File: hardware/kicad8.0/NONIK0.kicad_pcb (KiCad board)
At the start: 2 copper layers, 55 x 22 mm, 24 parts, among them J1 AVR-UPDI-3, J2 Qwiic/Stemma QT, J3 Test Pads, J4 Test Pads, SW1 SW_SPST, SW2 SW_Push, SW3 SW_Push, U1 LED_HCMS-2915, U2 ATtiny1604-SS, U3 AP3602A

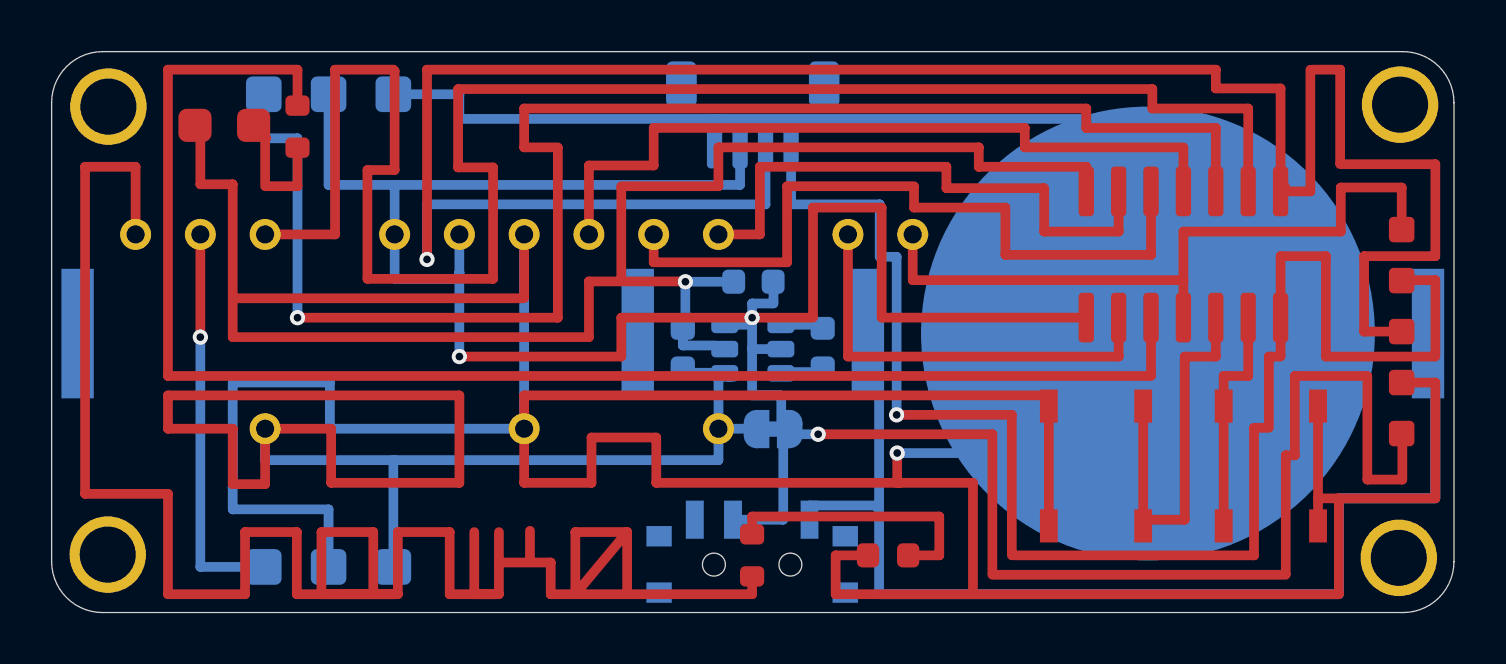
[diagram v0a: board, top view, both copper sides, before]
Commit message: pcb revisions
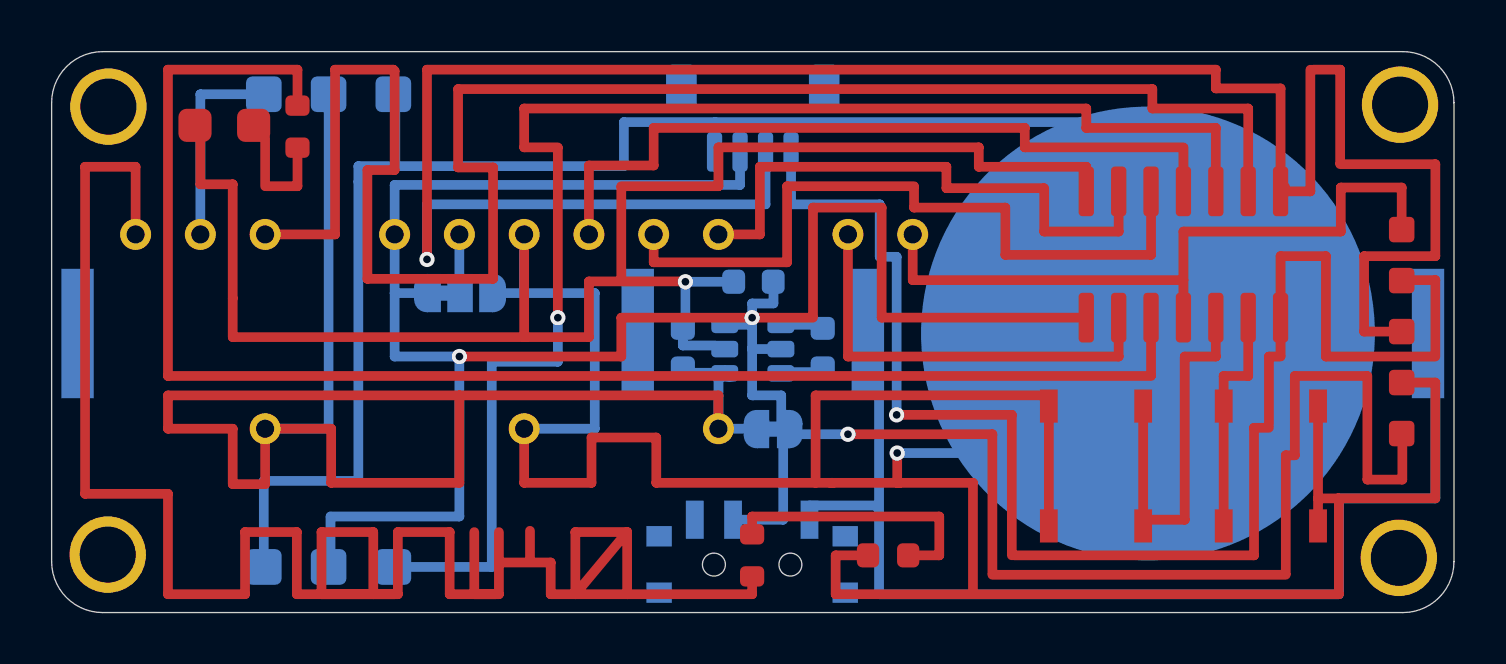
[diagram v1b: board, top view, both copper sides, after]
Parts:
- added JP2: SolderJumper_3_Bridged12, Jumper:SolderJumper-3_P1.3mm_Bridged12_RoundedPad1.0x1.5mm, B.Cu at (58.9, 27.1)
- moved J1 19.2 mm to (56.3, 37.8), turned to 180 degrees
- moved J4 18.5 mm to (51.2, 19.3)
- moved J2 0.13 mm to (70.4, 20.2)
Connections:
- J4 pad 2: GND -> Vled
- J4 pad 3: Vled -> GND
- U1 pad 21: VCC -> Net-(JP2-C)
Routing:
- net GND: track 272.5 -> 260.8 mm
- net OSC: track 15.5 -> 8.01 mm, vias 1 -> 0
- net VCC: track 127.3 -> 133.9 mm
- net UPDI: track 59.8 -> 56.1 mm
- net Vled: track 64.1 -> 66.6 mm
- net Net-(JP2-C): track 0.00 -> 2.35 mm
- net Net-(BZ1-+): track 5.33 -> 4.62 mm
